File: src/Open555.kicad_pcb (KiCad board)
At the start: 2 copper layers, 92.3 x 46.7 mm, 83 parts, among them J1 Conn_01x05_Pin, Q1 PNP, Q10 NPN, Q11 NPN, Q12 NPN, Q13 PNP, Q14 PNP, Q15 NPN, Q16 NPN, Q17 PNP, Q18 PNP, Q19 NPN, Q2 PNP, Q20 NPN, Q21 NPN, Q22 NPN, Q3 PNP, Q4 PNP, Q5 PNP, Q6 PNP, Q7 PNP, Q8 NPN, Q9 NPN, SW1 SW_Push

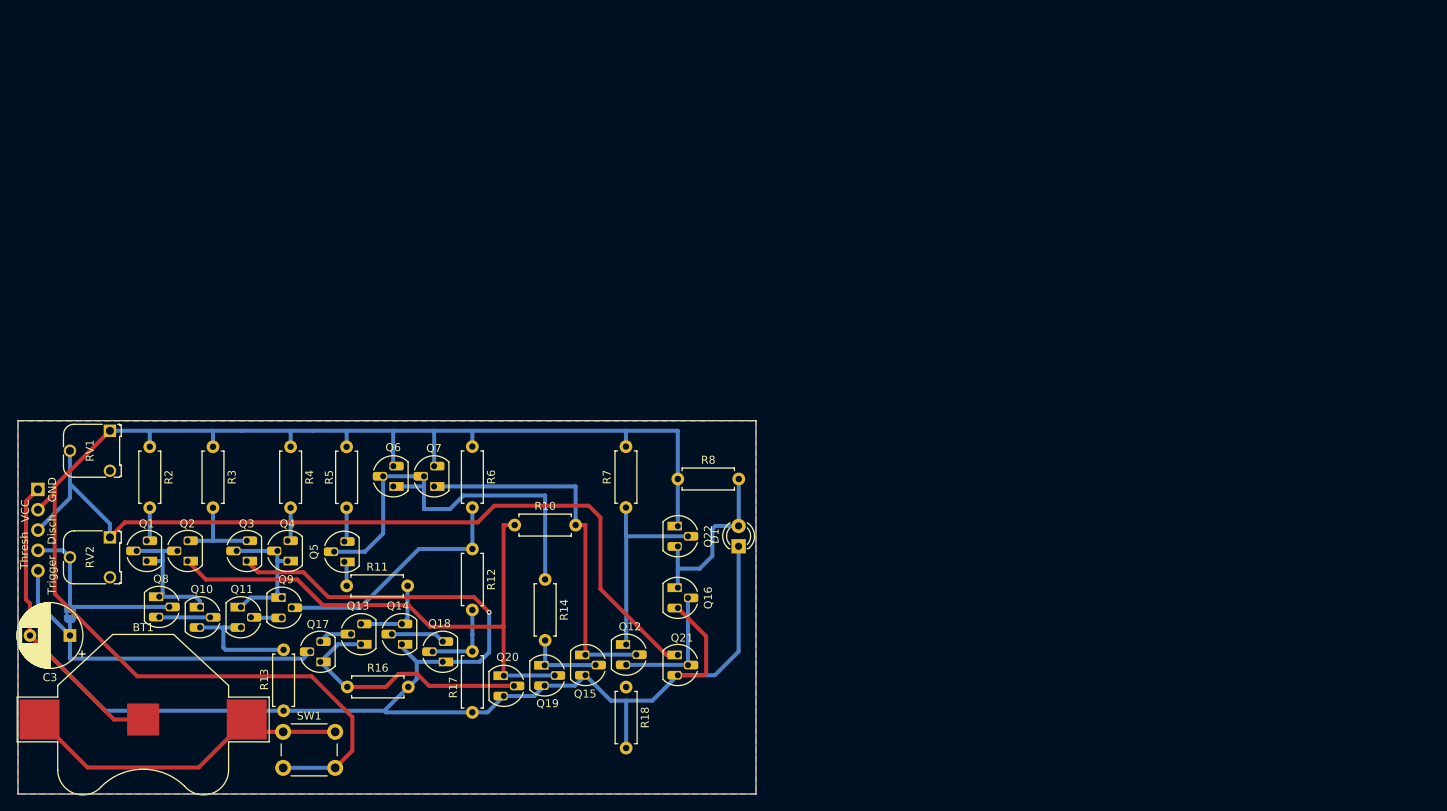
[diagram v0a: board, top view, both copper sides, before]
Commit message: Final revision
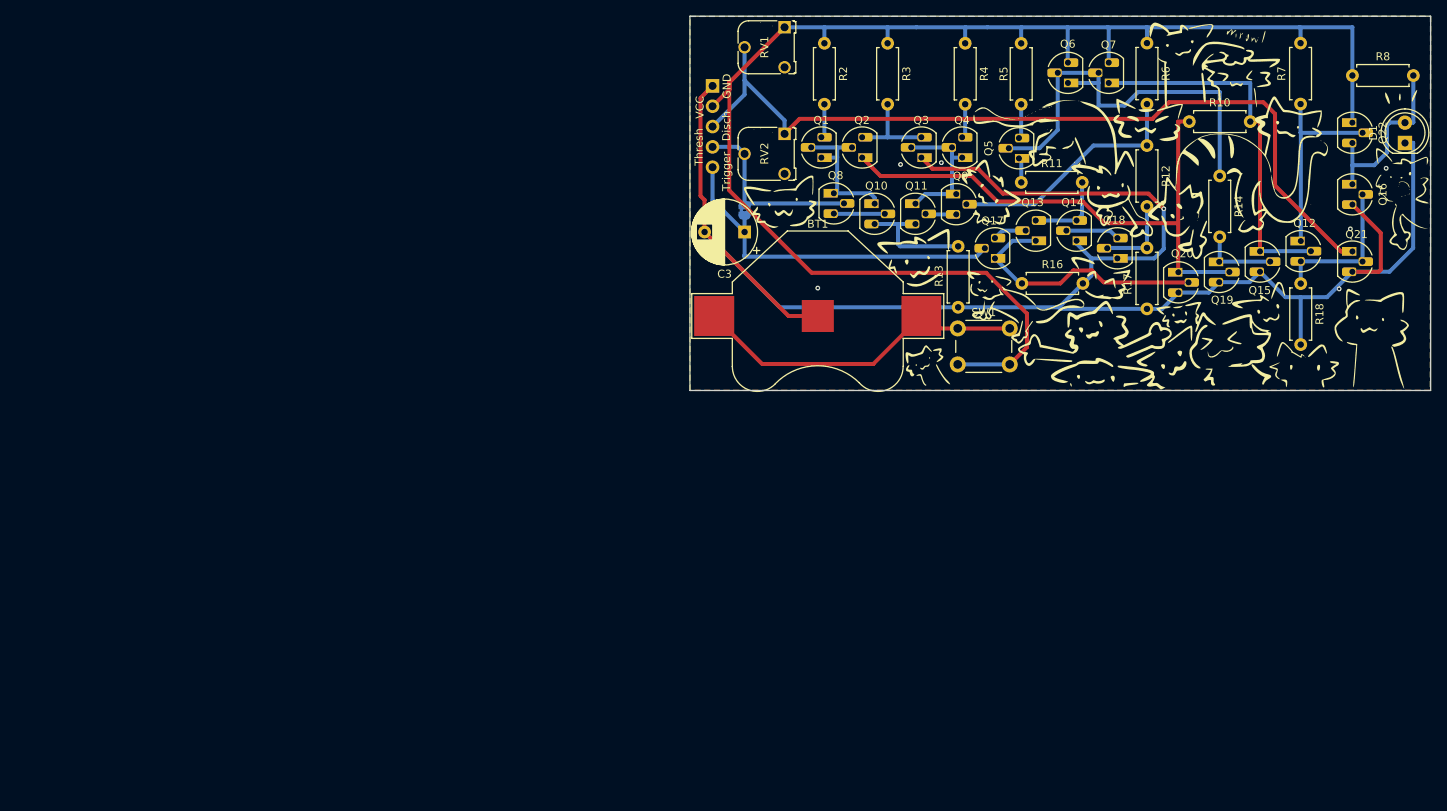
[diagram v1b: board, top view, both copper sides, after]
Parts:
- added G***: LOGO, LOGO, F.Cu at (149.2, 95.1)
- D1: footprint LED_THT:LED_D3.0mm -> LED_THT:LED_D5.0mm
- R10, R11, R12, R14, R17, R18, R2, R4, R5, R6: value R -> 4.7k
- R13: value R -> 10k
- R16: value R -> 100k
- R3, R7, R8: value R -> 100
- moved G*** 98.3 mm to (169.3, 95.4)
- moved G*** 98.3 mm to (148.3, 92.5)
- moved G*** 98.3 mm to (141.4, 100.7)
- moved G*** 98.3 mm to (169.1, 103.7)
- moved G*** 98.3 mm to (151.6, 98.5)
- moved G*** 98.3 mm to (179.3, 101.1)
- moved G*** 98.3 mm to (174.2, 102.4)
- moved G*** 98.3 mm to (132.4, 90.6)
- moved G*** 98.3 mm to (179.4, 109.0)
- moved R3 98.3 mm to (127.8, 75.1)
- moved BT1 98.3 mm to (119.1, 109.2)
- moved G*** 98.3 mm to (160.2, 104.5)
- moved G*** 98.3 mm to (185.8, 102.4)
- moved G*** 98.3 mm to (120.9, 95.1)
- moved G*** 98.3 mm to (127.8, 78.9)
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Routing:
- net Net-(Q12-E): track 16.1 -> 18.9 mm
- net GND: track 226.6 -> 227.6 mm, vias 1 -> 7
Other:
- board size 92.3 x 46.7 mm -> 92.6 x 46.8 mm
